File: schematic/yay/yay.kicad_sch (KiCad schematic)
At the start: 18 parts, among them SW1 SW_SPDT, SW2 SW_Push, SW3 SW_SPDT, SW4 SW_Push, SW6 SW_SPDT, U1 xiao esp32-s3 sense, U2 IP2312 Li-Ion charger 4.2V, U3 xiao esp32-s3 sense, U4 IP2312 Li-Ion charger 4.2V

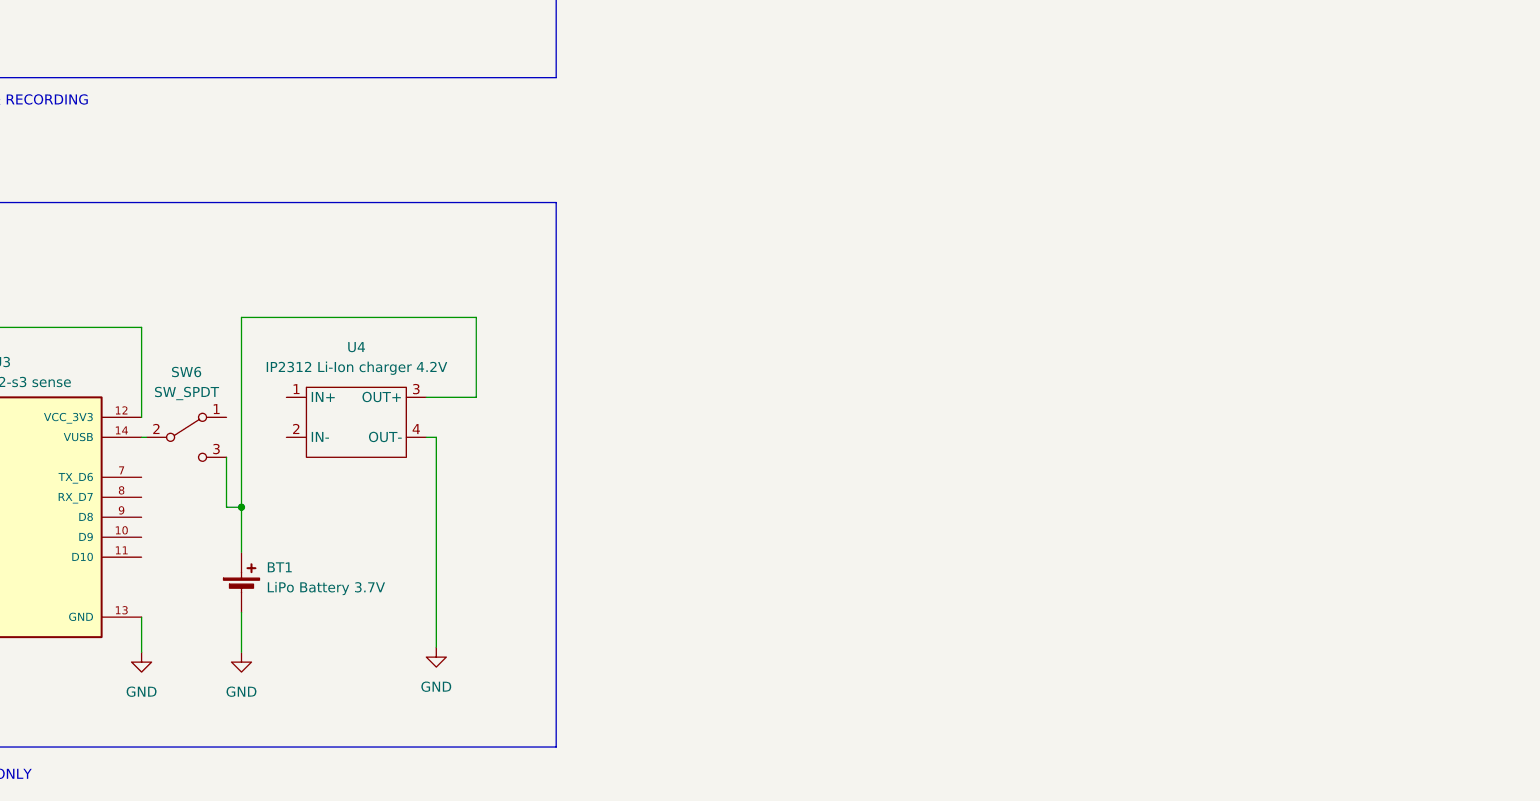
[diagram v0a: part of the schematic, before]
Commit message: more 3d updates
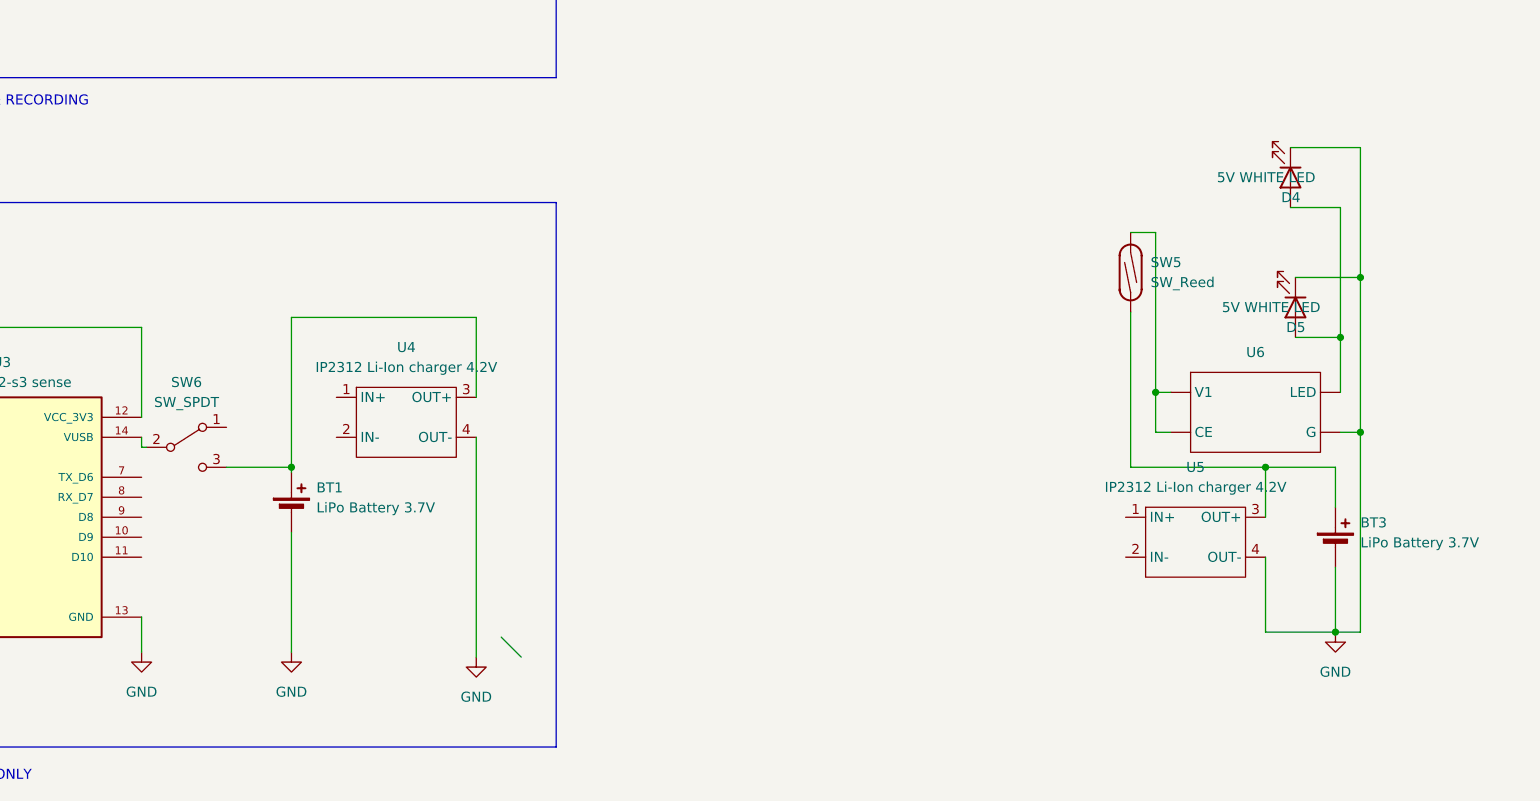
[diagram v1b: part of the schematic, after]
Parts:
- added BT3: LiPo Battery 3.7V, symbol Device:Battery_Cell
- added D4, D5: 5V WHITE LED, symbol Device:LED
- added SW5: SW_Reed, symbol Switch:SW_Reed
- added U5: IP2312 Li-Ion charger 4.2V, Battery:BatteryHolder_Keystone_2460_1xAA, symbol li-ion_charger:IP2312_Li-Ion_charger
- added U6: ~, symbol LED_vustom:LD06AJSA_led_driver
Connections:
- net GND: now also BT3.2 (-), D4.1 (K), D5.1 (K), U5.4 (OUT-), U6. (V1)
- new net: BT3.1 (+), SW5.2, U5.3 (OUT+)
- new net: SW5.1, U6. (V1)
- new net: D4.2 (A), D5.2 (A), U6. (V1)
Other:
- moved on the sheet: BT1, SW6, U4
